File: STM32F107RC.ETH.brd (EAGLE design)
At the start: 160 x 100 mm, 28 parts, among them J1 HR911105A, Q1 8MHz, U1 LAN8720A-CP, U2 STM32F107RCT6, X1 CB3LV-3I-74M2500

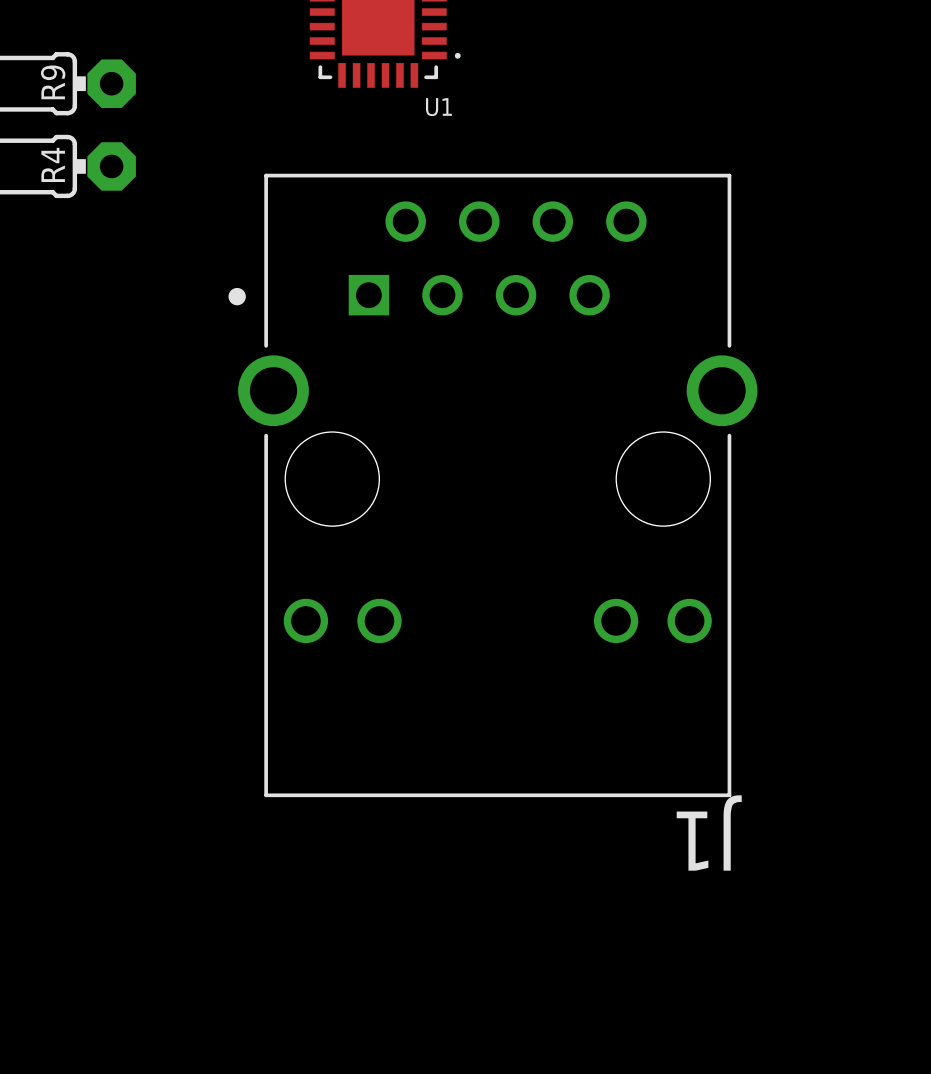
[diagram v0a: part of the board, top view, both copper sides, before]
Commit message: Add files via upload
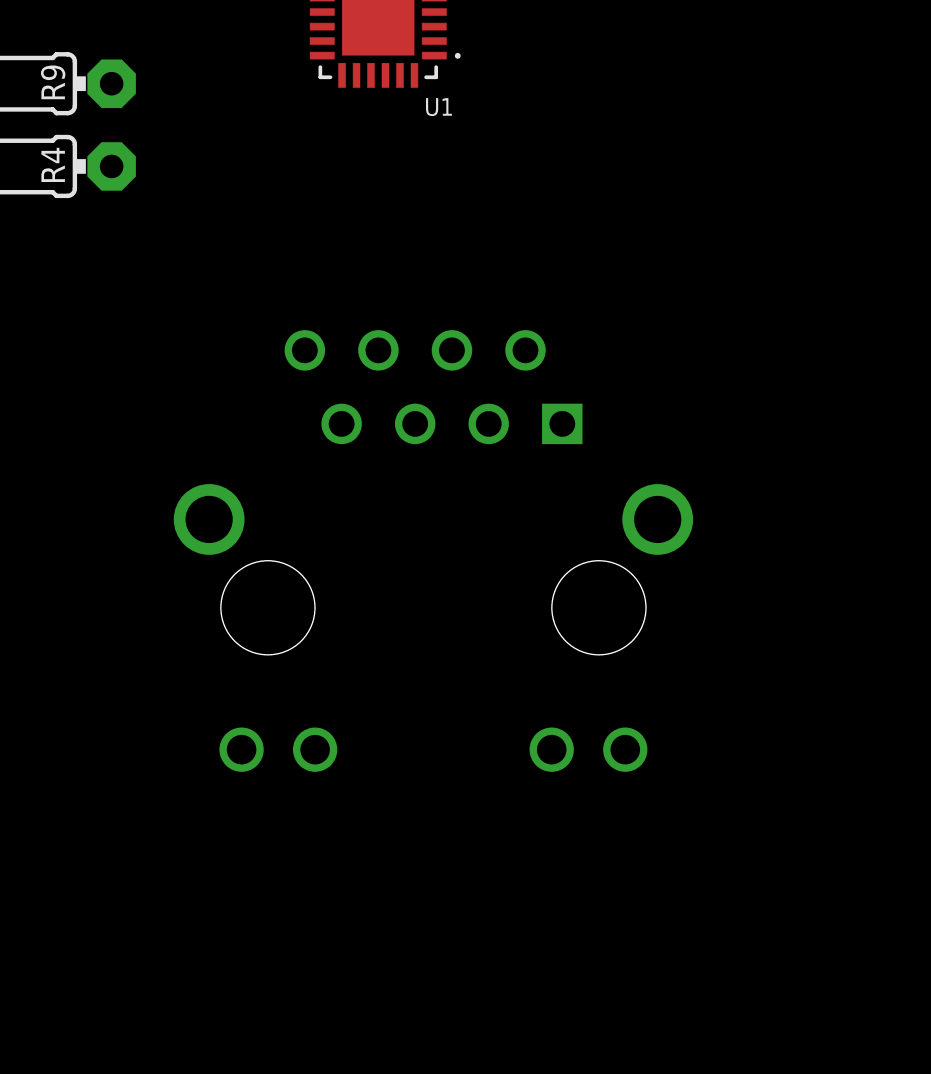
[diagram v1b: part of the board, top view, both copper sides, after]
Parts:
- moved J1 4.97 mm to (92.4, 27.0), flipped to the bottom
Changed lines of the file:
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@@
 <attribute name="SPICEPREFIX" value="C" x="44.45" y="46.355" size="1.778" layer="27" rot="R90" display="off"/>
 </element>
-<element name="J1" library="HR911105A" package="HANRUN_HR911105A" value="HR911105A" x="94.615" y="31.4325" rot="R180">
-<attribute name="PACKAGE" value="None" x="94.615" y="31.4325" size="1.778" layer="27" rot="R180" display="off"/>
-<attribute name="MP" value="HR911105A" x="94.615" y="31.4325" size="1.778" layer="27" rot="R180" display="off"/>
-<attribute name="AVAILABILITY" value="Unavailable" x="94.615" y="31.4325" size="1.778" layer="27" rot="R180" display="off"/>
-<attribute name="PRICE" value="None" x="94.615" y="31.4325" size="1.778" layer="27" rot="R180" display="off"/>
-<attribute name="DESCRIPTION" value=" DIP RJ45 Connector; " x="94.615" y="31.4325" size="1.778" layer="27" rot="R180" display="off"/>
-<attribute name="MF" value="HanRun" x="94.615" y="31.4325" size="1.778" layer="27" rot="R180" display="off"/>
+<element name="J1" library="HR911105A" package="HANRUN_HR911105A" value="HR911105A" x="92.3925" y="26.9875" rot="MR180">
+<attribute name="PACKAGE" value="None" x="92.3925" y="26.9875" size="1.778" layer="28" rot="MR180" display="off"/>
+<attribute name="MP" value="HR911105A" x="92.3925" y="26.9875" size="1.778" layer="28" rot="MR180" display="off"/>
+<attribute name="AVAILABILITY" value="Unavailable" x="92.3925" y="26.9875" size="1.778" layer="28" rot="MR180" display="off"/>
+<attribute name="PRICE" value="None" x="92.3925" y="26.9875" size="1.778" layer="28" rot="MR180" display="off"/>
+<attribute name="DESCRIPTION" value=" DIP RJ45 Connector; " x="92.3925" y="26.9875" size="1.778" layer="28" rot="MR180" display="off"/>
+<attribute name="MF" value="HanRun" x="92.3925" y="26.9875" size="1.778" layer="28" rot="MR180" display="off"/>
 </element>
 <element name="J2" library="SparkFun-Connectors" package="1X01_OFFSET" value="" x="108.2675" y="70.8025" rot="R270"/>
@@
 <wire x1="44.45" y1="47.755" x2="104.58" y2="55.245" width="0" layer="19" extent="1-1"/>
 <wire x1="39.37" y1="46.99" x2="44.45" y2="47.755" width="0" layer="19" extent="1-1"/>
-<wire x1="99.055" y1="40.3225" x2="73.66" y2="42.2275" width="0" layer="19" extent="1-1"/>
+<wire x1="87.9525" y1="35.8775" x2="73.66" y2="42.2275" width="0" layer="19" extent="1-1"/>
 </signal>
 <signal name="N$6">
@@
 <contactref element="J1" pad="12"/>
 <wire x1="90.7375" y1="49.2425" x2="108.78" y2="60.325" width="0" layer="19" extent="1-1"/>
-<wire x1="93.975" y1="40.3225" x2="90.7375" y2="49.2425" width="0" layer="19" extent="1-1"/>
-<wire x1="95.245" y1="37.7825" x2="93.975" y2="40.3225" width="0" layer="19" extent="1-1"/>
-<wire x1="101.24" y1="26.5325" x2="95.245" y2="37.7825" width="0" layer="19" extent="1-1"/>
-<wire x1="87.99" y1="26.5325" x2="101.24" y2="26.5325" width="0" layer="19" extent="1-1"/>
+<wire x1="93.0325" y1="35.8775" x2="90.7375" y2="49.2425" width="0" layer="19" extent="1-1"/>
+<wire x1="91.7625" y1="33.3375" x2="93.0325" y2="35.8775" width="0" layer="19" extent="1-1"/>
+<wire x1="85.7675" y1="22.0875" x2="91.7625" y2="33.3375" width="0" layer="19" extent="1-1"/>
+<wire x1="99.0175" y1="22.0875" x2="85.7675" y2="22.0875" width="0" layer="19" extent="1-1"/>
 <wire x1="60.325" y1="48.5775" x2="90.7375" y2="49.2425" width="0" layer="19" extent="1-1"/>
 <wire x1="60.325" y1="51.7525" x2="60.325" y2="48.5775" width="0" layer="19" extent="1-1"/>
@@
 <contactref element="U1" pad="21"/>
 <contactref element="J1" pad="1"/>
-<wire x1="90.165" y1="37.7825" x2="90.2375" y2="45.3725" width="0" layer="19" extent="1-1"/>
+<wire x1="96.8425" y1="33.3375" x2="90.2375" y2="45.3725" width="0" layer="19" extent="1-1"/>
 </signal>
 <signal name="N$28">
 <contactref element="U1" pad="20"/>
 <contactref element="J1" pad="2"/>
-<wire x1="91.435" y1="40.3225" x2="89.7375" y2="45.3725" width="0" layer="19" extent="1-1"/>
+<wire x1="95.5725" y1="35.8775" x2="89.7375" y2="45.3725" width="0" layer="19" extent="1-1"/>
 </signal>
 <signal name="N$29">
 <contactref element="U1" pad="23"/>
 <contactref element="J1" pad="3"/>
-<wire x1="92.705" y1="37.7825" x2="91.2375" y2="45.3725" width="0" layer="19" extent="1-1"/>
+<wire x1="94.3025" y1="33.3375" x2="91.2375" y2="45.3725" width="0" layer="19" extent="1-1"/>
 </signal>
 <signal name="N$31">
 <contactref element="U1" pad="22"/>
 <contactref element="J1" pad="6"/>
-<wire x1="96.515" y1="40.3225" x2="90.7375" y2="45.3725" width="0" layer="19" extent="1-1"/>
+<wire x1="90.4925" y1="35.8775" x2="90.7375" y2="45.3725" width="0" layer="19" extent="1-1"/>
 </signal>
 <signal name="LED2">
 <contactref element="U1" pad="2"/>
 <contactref element="J1" pad="11"/>
-<wire x1="98.7" y1="26.5325" x2="92.4225" y2="46.5575" width="0" layer="19" extent="1-1"/>
+<wire x1="88.3075" y1="22.0875" x2="92.4225" y2="46.5575" width="0" layer="19" extent="1-1"/>
 </signal>
 <signal name="LED1">
 <contactref element="U1" pad="3"/>
 <contactref element="J1" pad="10"/>
-<wire x1="90.53" y1="26.5325" x2="92.4225" y2="47.0575" width="0" layer="19" extent="1-1"/>
+<wire x1="96.4775" y1="22.0875" x2="92.4225" y2="47.0575" width="0" layer="19" extent="1-1"/>
 </signal>
 </signals>
